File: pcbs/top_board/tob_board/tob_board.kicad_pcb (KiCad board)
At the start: 2 copper layers, 40 x 40 mm, 9 parts, among them J1 LEDFrontRight, J2 LEDRearRight, J3 LEDFrontLeft, J4 LEDRearLeft, J5 Motor, J6 Motor1, J7 Motor2

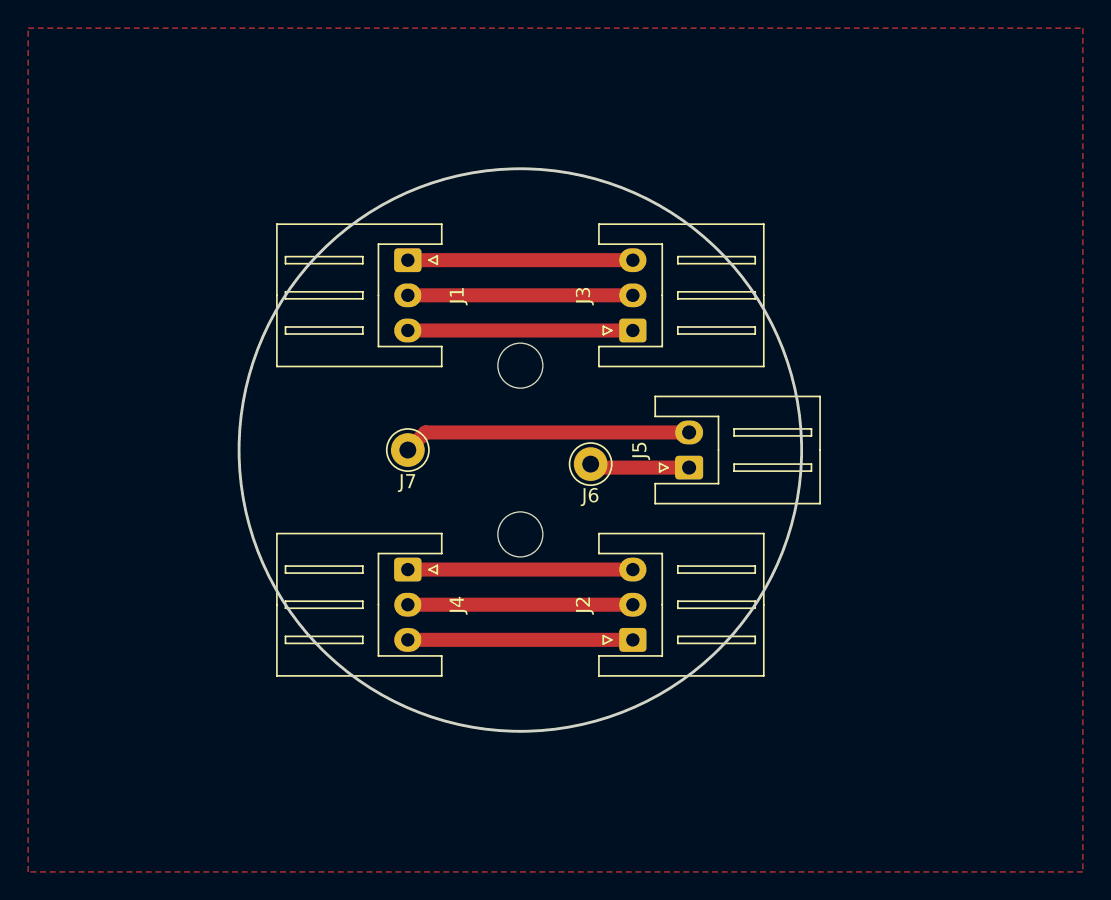
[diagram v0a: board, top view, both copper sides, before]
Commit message: board update
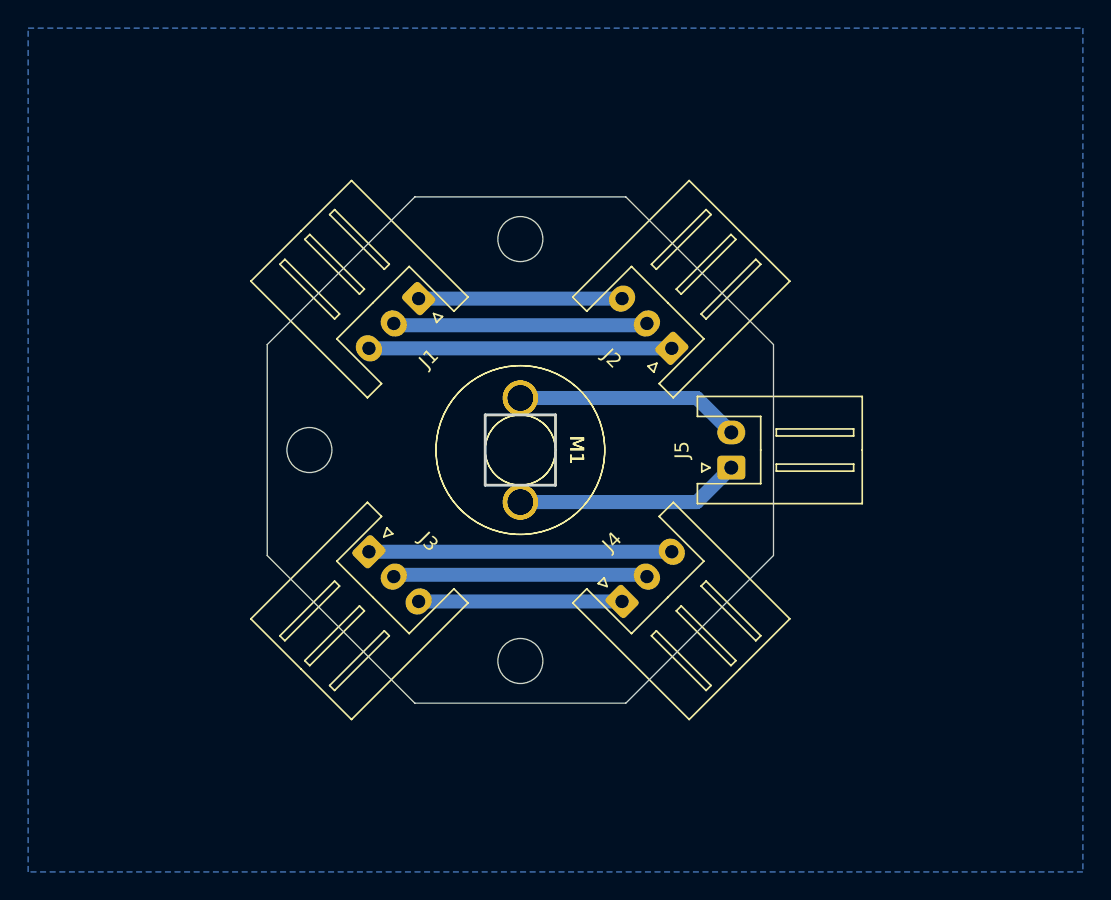
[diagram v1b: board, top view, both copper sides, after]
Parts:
- removed J6: Motor1, Connector_Pin:Pin_D1.0mm_L10.0mm_LooseFit
- removed J7: Motor2, Connector_Pin:Pin_D1.0mm_L10.0mm_LooseFit
- removed the REF** at (180.0, 76.0)
- removed the REF** at (180.0, 64.0)
- added M1 (x2): Motor_DC, topMotor:topMotor, F.Cu at (180.0, 70.0)
- added REF**: MountingHole_3.2mm_M3, MountingHole:MountingHole_3.2mm_M3, F.Cu at (180.0, 85.0)
- added REF**: MountingHole_3.2mm_M3, MountingHole:MountingHole_3.2mm_M3, F.Cu at (180.0, 55.0)
- added REF**: MountingHole_3.2mm_M3, MountingHole:MountingHole_3.2mm_M3, F.Cu at (165.0, 70.0)
- moved J2 19.8 mm to (190.8, 62.8), turned to 135 degrees
- moved J1 15.4 mm to (172.8, 59.2), turned to -135 degrees
- moved J3 3.04 mm to (169.2, 77.2), turned to -45 degrees
- moved J5 3.00 mm to (195.0, 71.2)
- moved J4 2.84 mm to (187.2, 80.8), turned to 45 degrees
- renumbered J3 to J1, J1 to J2, J4 to J3, J2 to J4
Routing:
- net Net-(J5-Pin_1): track 7.10 -> 16.0 mm
- net Net-(J3-Pin_1): track 16.0 -> 21.5 mm
- net Net-(J1-Pin_3): track 16.0 -> 21.5 mm
- net Net-(J5-Pin_2): track 20.5 -> 16.0 mm
- net Net-(J3-Pin_2): track 16.0 -> 18.5 mm
- net Net-(J1-Pin_2): track 16.0 -> 18.1 mm
- net Net-(J3-Pin_3): track 16.0 -> 14.5 mm
- net Net-(J1-Pin_1): track 16.0 -> 14.5 mm
- added copper zone on B.Cu, net (none)
- removed copper zone on F.Cu, net (none)
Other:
- board size 40 x 40 mm -> 36 x 36 mm
